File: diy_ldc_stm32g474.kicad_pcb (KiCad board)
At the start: 4 copper layers, 50.2 x 40 mm, 91 parts, among them J1 USB_B_Micro, J10 Conn_02x03_Odd_Even, J12 Conn_01x04, J13 Conn_01x05, J2 Conn_01x02, J3 Conn_01x03, J4 Conn_01x04, J6 Conn_Coaxial, J7 Conn_Coaxial, J8 Conn_Coaxial, J9 Conn_Coaxial, U1 XC6206PxxxMR, U2 STM32G431CBUx, U3 SN74LVC2G14DBV, U4 SN74LVC2G14DBV, U5 TPH2502-SR, U6 TLV2333IDR, U7 TPS61040DBV, U8 OPA2188AIDR, Y1 24MHz, 9pF

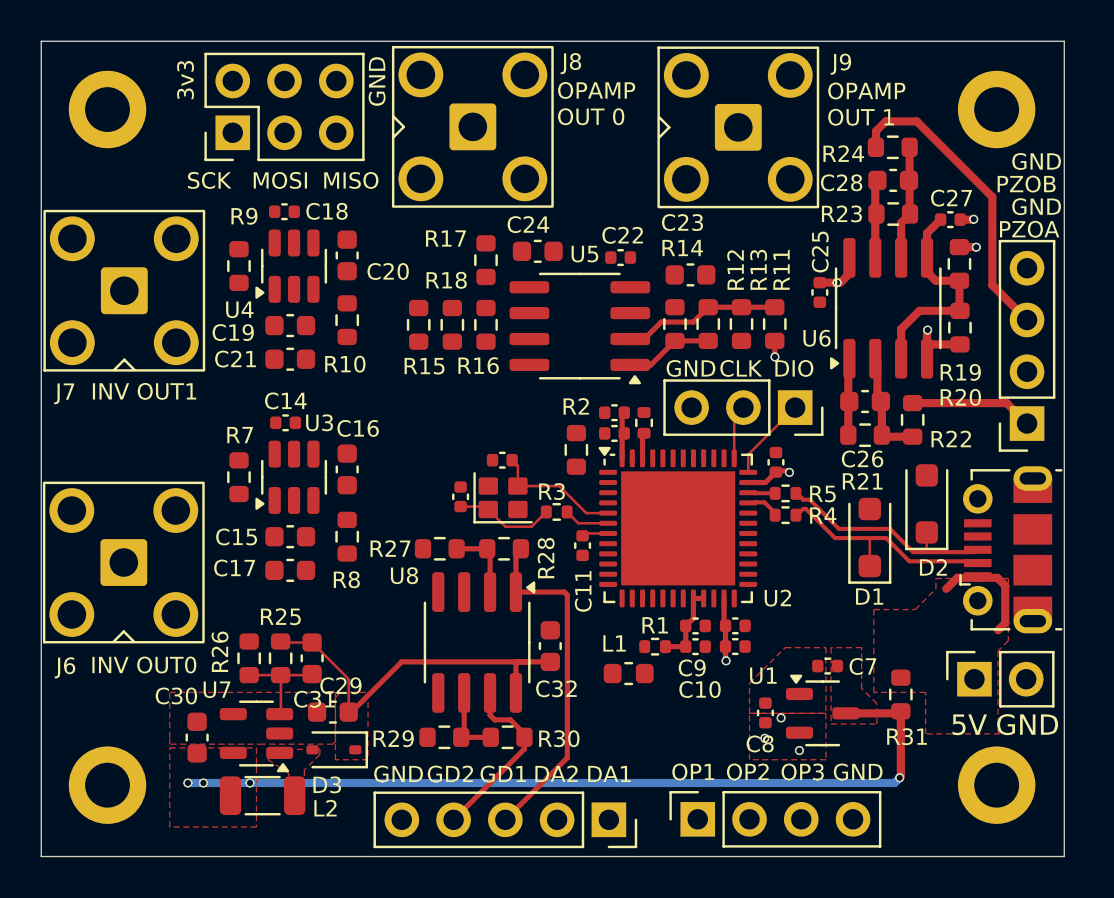
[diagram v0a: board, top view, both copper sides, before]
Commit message: Preliminary routing done
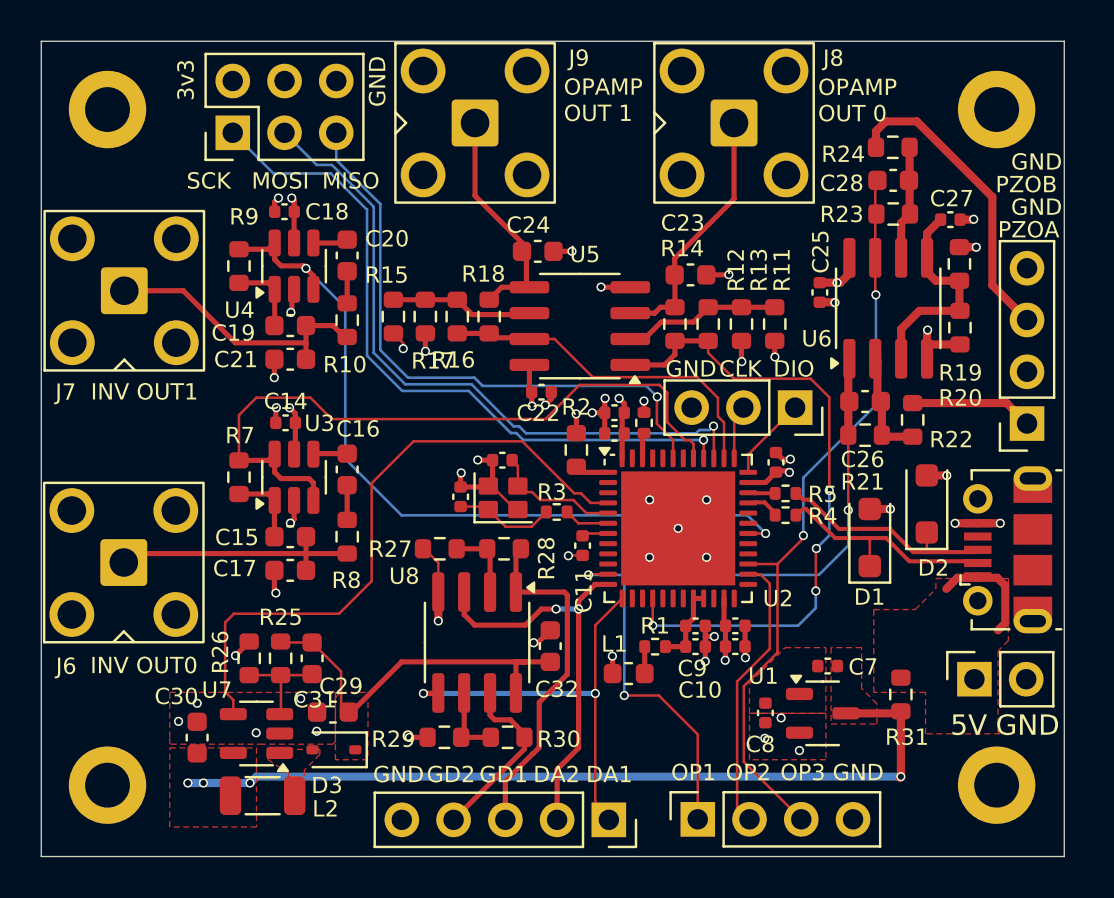
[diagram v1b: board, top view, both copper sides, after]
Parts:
- moved J9 12.9 mm to (161.3, 64.0)
- moved J8 12.8 mm to (174.0, 64.0)
- moved C22 7.66 mm to (164.5, 77.2)
- moved R17 4.07 mm to (158.8, 73.5), turned to 90 degrees
- moved R18 1.85 mm to (162.0, 73.5)
- moved R16 1.47 mm to (160.4, 73.5)
- moved R15 1.31 mm to (157.3, 73.5)
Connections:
- J10 pad 1: /MCU/SPI3_SCK -> /MCU/SPI3_MISO
- J10 pad 3: /MCU/SPI3_MOSI -> /MCU/SPI3_SCK
- J10 pad 5: /MCU/SPI3_MISO -> /MCU/SPI3_MOSI
- J13 pad 1: /MCU/piezo_drive/dac1_out1 -> /MCU/dac1_out2
- J13 pad 2: /MCU/piezo_drive/dac1_out2 -> /MCU/dac1_out1
- J4 pad 2: /MCU/opamp2_vinp -> /MCU/opamp3_vinp
- J4 pad 3: /MCU/opamp3_vinp -> /MCU/opamp2_vinp
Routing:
- net /MCU/TIM4_ETR: track 0.00 -> 38.7 mm, vias 0 -> 2
- net GND: track 4.32 -> 42.5 mm, vias 2 -> 43
- net /MCU/opamp1_vinp: track 3.77 -> 40.1 mm, vias 0 -> 3
- net /MCU/TIM3_ETR: track 0.00 -> 34.5 mm
- net /MCU/SPI3_MISO: track 0.00 -> 34.4 mm, vias 0 -> 1
- net /MCU/SPI3_SCK: track 0.00 -> 33.1 mm, vias 0 -> 1
- net /MCU/opamp2_vinp: track 3.85 -> 36.7 mm, vias 0 -> 2
- net /MCU/BOOST_EN: track 0.00 -> 31.2 mm
- net /MCU/SPI3_MOSI: track 0.00 -> 29.4 mm, vias 0 -> 1
- net /MCU/TIM1_ETR: track 4.31 -> 32.4 mm, vias 0 -> 4
- net /MCU/dac1_out2: track 0.00 -> 20.9 mm, vias 0 -> 2
- net /MCU/dac1_out1: track 0.00 -> 20.2 mm, vias 0 -> 2
- net /MCU/TIM2_ETR: track 0.00 -> 17.2 mm
- net Net-(J7-In): track 0.00 -> 13.9 mm
- net /MCU/opamp3_vinp: track 0.00 -> 13.7 mm
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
